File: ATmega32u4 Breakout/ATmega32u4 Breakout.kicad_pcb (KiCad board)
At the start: 2 copper layers, 6 parts, among them J1 Conn_01x22_Male, J2 Conn_01x22_Male, U1 ATmega32U4-AU, Y1 16MHz

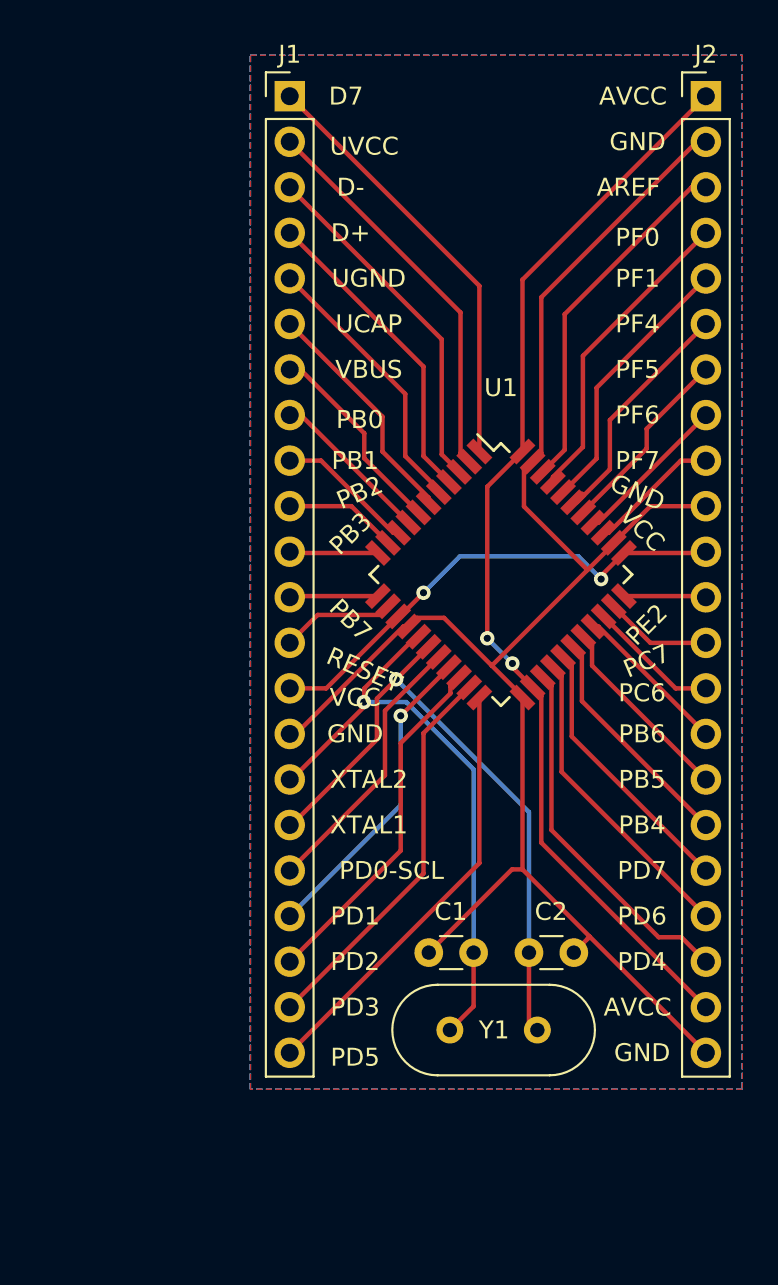
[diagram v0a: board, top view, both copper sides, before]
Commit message: Lots of work over the weekend.
Nearly done, gerber files made too.  I think it's ready to be turned into PCB.
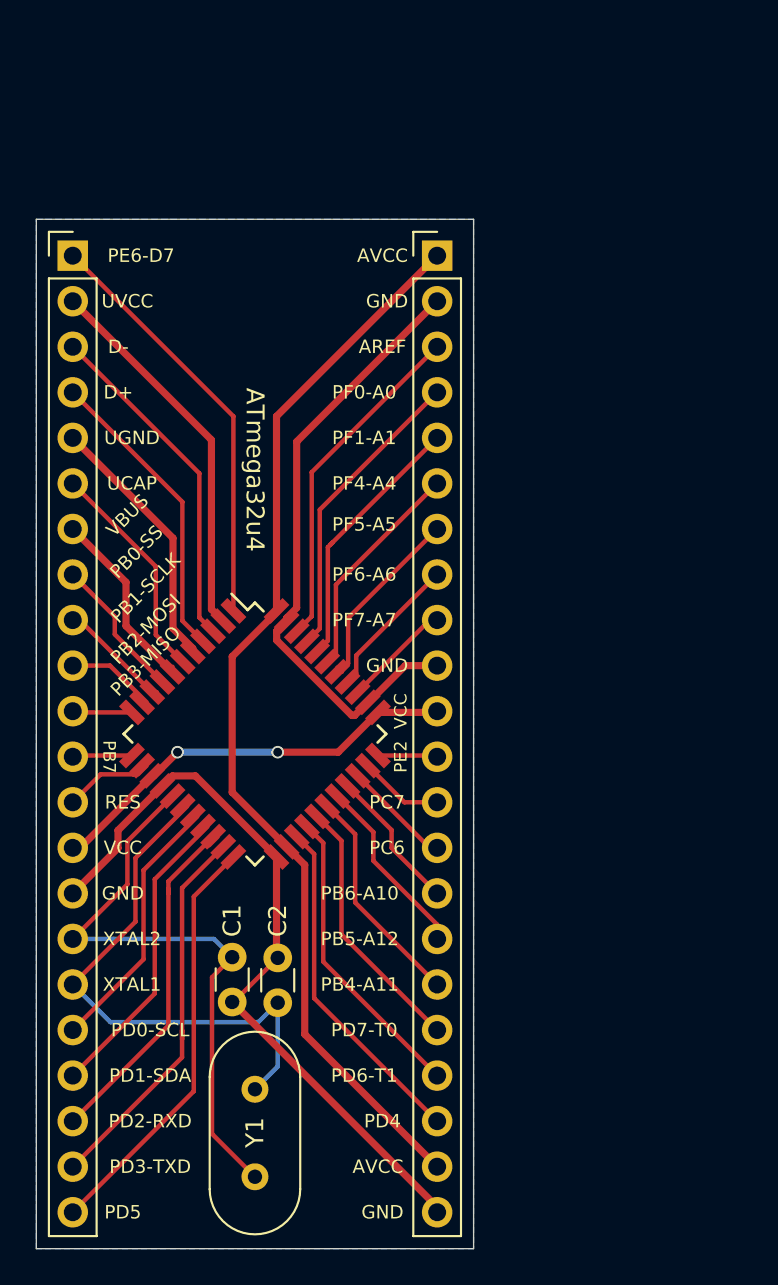
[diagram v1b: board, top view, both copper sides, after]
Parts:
- moved J2 17.4 mm to (152.1, 71.1)
- moved U1 16.3 mm to (142.0, 97.8)
- moved Y1 16.1 mm to (142.0, 117.6), turned to 270 degrees
- moved J1 15.0 mm to (131.8, 71.1)
- moved C2 14.3 mm to (143.3, 112.8), turned to 90 degrees
- moved C1 13.5 mm to (140.7, 110.2), turned to 270 degrees
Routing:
- net GND: track 95.5 -> 76.7 mm
- net XTAL1: track 36.0 -> 31.4 mm, vias 2 -> 1
- net VCC: track 27.5 -> 23.5 mm
- net PB1: track 7.71 -> 5.97 mm
- net PB3: track 4.95 -> 3.33 mm
- net PB7: track 4.94 -> 3.33 mm
- net PE2: track 4.60 -> 3.08 mm
- net PB2: track 6.33 -> 4.97 mm
- net PD4: track 20.4 -> 19.1 mm
- net PC7: track 5.98 -> 4.71 mm
- net PC6: track 7.37 -> 6.10 mm
- net PF4: track 13.8 -> 12.6 mm
- net PF7: track 7.37 -> 6.26 mm
- net PB0: track 9.10 -> 8.06 mm
- net AREF: track 20.1 -> 19.1 mm
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- removed copper zone on F.Cu, net GND
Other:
- board outline added: 24.4 x 57.4 mm
- net class Power added: clearance 0.2, trace_width 0.4, via_dia 0.7, via_drill 0.5
- rule pad_to_mask_clearance: 0 -> 0.0508
- board text added: "ATmega32u4"
- board text added: "PB0-SS"
- board text added: "PB1-SCLK"
- board text added: "PB2-MOSI"
- board text added: "PB3-MISO"
- board text added: "PB4-A11"
- board text added: "PB5-A12"
- board text added: "PB6-A10"
- board text added: "PD1-SDA"
- board text added: "PD2-RXD"
- board text added: "PD3-TXD"
- board text added: "PD6-T1"
- board text added: "PD7-T0"
- board text added: "PE6-D7"
- board text added: "PF0-A0"
- board text added: "PF1-A1"
- board text added: "PF4-A4"
- board text added: "PF5-A5"
- board text added: "PF6-A6"
- board text added: "PF7-A7"
- board text added: "RES"
- board text added: "SRT0001"
- board text removed: "D7"
- board text removed: "PB0"
- board text removed: "PB1"
- board text removed: "PB2"
- board text removed: "PB3"
- board text removed: "PB4"
- board text removed: "PB5"
- board text removed: "PB6"
- board text removed: "PD1"
- board text removed: "PD2"
- board text removed: "PD3"
- board text removed: "PD6"
- board text removed: "PD7"
- board text removed: "PF0"
- board text removed: "PF1"
- board text removed: "PF4"
- board text removed: "PF5"
- board text removed: "PF6"
- board text removed: "PF7"
- board text removed: "RESET"
